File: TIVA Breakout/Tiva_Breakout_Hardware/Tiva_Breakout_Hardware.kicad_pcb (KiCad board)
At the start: 2 copper layers, 141.4 x 70.3 mm, 67 parts, among them U1 TM4C129E_Launchpad

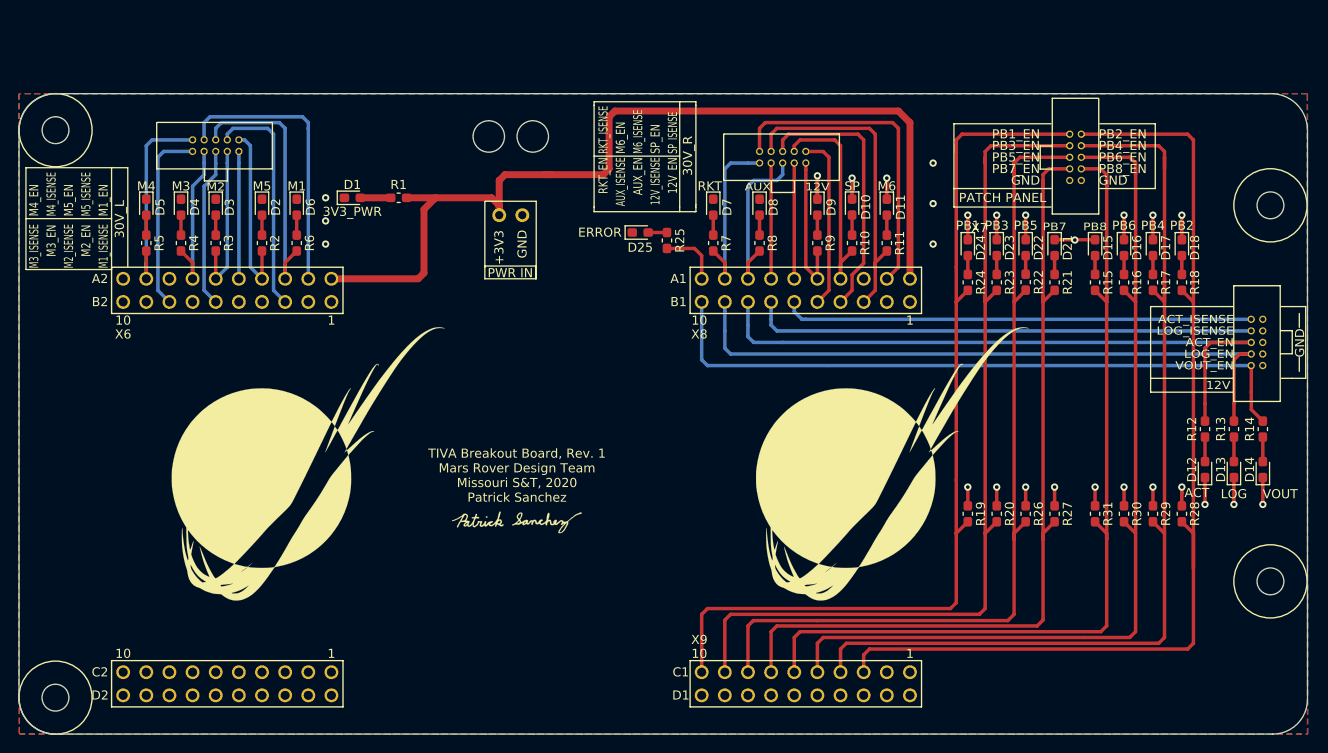
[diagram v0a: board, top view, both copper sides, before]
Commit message: Ready for Board Review, questions about PB#
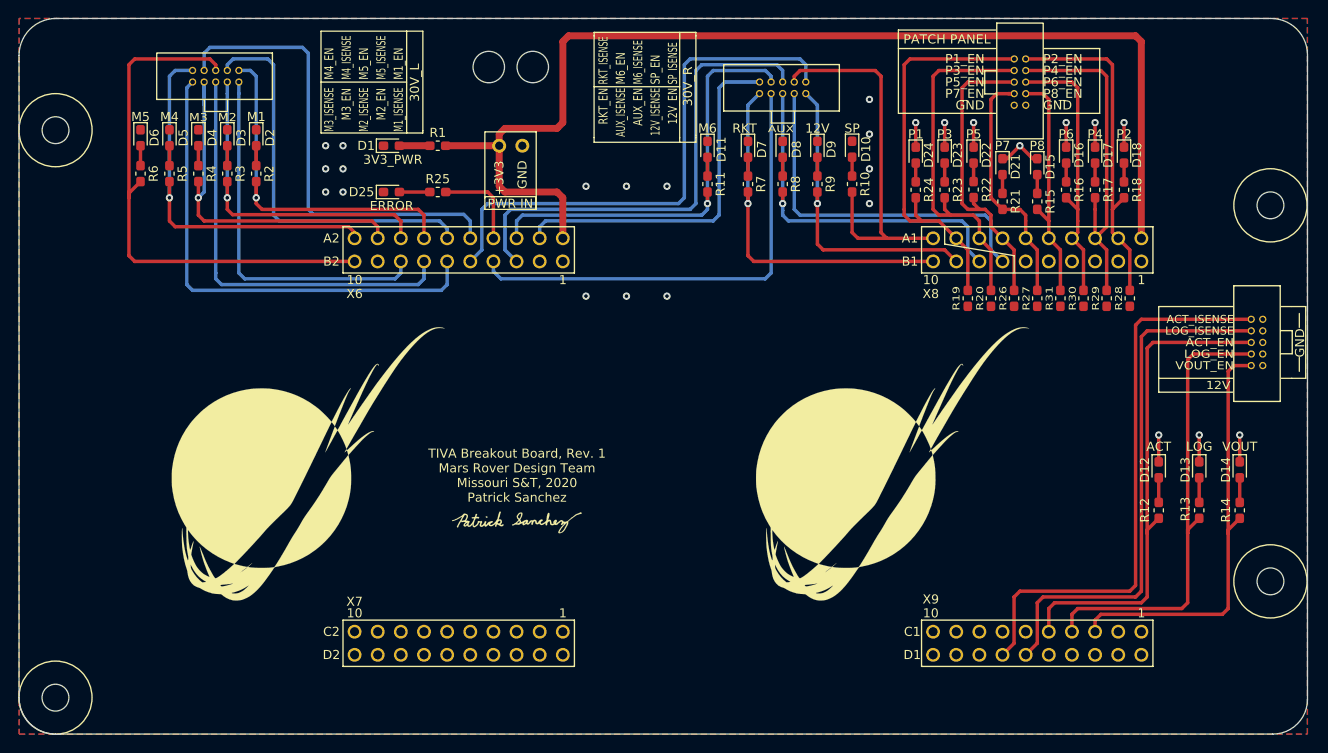
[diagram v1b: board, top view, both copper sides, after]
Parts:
- moved D25 27.7 mm to (125.4, 86.1)
- moved U1 25.8 mm to (209.0, 89.9)
- moved R25 25.7 mm to (130.5, 86.1), turned to 0 degrees
- moved R28 24.3 mm to (206.5, 97.8), turned to 90 degrees
- moved R29 24.2 mm to (203.9, 97.8), turned to 90 degrees
- moved R30 24.1 mm to (201.4, 97.8), turned to 90 degrees
- moved R31 24.0 mm to (198.8, 97.8), turned to 90 degrees
- moved R27 23.7 mm to (196.3, 97.8), turned to 90 degrees
- moved R26 23.7 mm to (193.8, 97.8), turned to 90 degrees
- moved R20 23.7 mm to (191.2, 97.8), turned to 90 degrees
- moved R19 23.7 mm to (188.7, 97.8), turned to 90 degrees
- moved R11 20.7 mm to (160.1, 85.2)
- moved D11 20.7 mm to (160.1, 81.4)
- moved D6 18.8 mm to (97.9, 80.2)
- moved R6 18.8 mm to (97.9, 84.1)
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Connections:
- U1 pad PA5: Net-(U1-PadPA5) -> M5_EN
- U1 pad PA6: ACT_EN -> AUX_EN
- U1 pad PB2: RKT_EN -> PB1_EN
- U1 pad PB3: ERROR -> SP_EN
- U1 pad PB4: M5_ISENSE -> M6_ISENSE
- U1 pad PB5: Net-(U1-PadPB5) -> AUX_ISENSE
- U1 pad PC4: Net-(U1-PadPC4) -> PB4_EN
- U1 pad PC5: SP_EN -> PB6_EN
- U1 pad PC6: 12V_EN -> PB8_EN
- U1 pad PC7: AUX_EN -> PB3_EN
- U1 pad PD0: Net-(U1-PadPD0) -> ACT_ISENSE
- U1 pad PD1: Net-(U1-PadPD1) -> LOG_ISENSE
- U1 pad PD2: M4_ISENSE -> RKT_ISENSE
- U1 pad PD3: AUX_ISENSE -> PB5_EN
- U1 pad PD4: M1_ISENSE -> M4_ISENSE
- U1 pad PD5: M2_EN -> M5_ISENSE
- U1 pad PD7: LOG_ISENSE -> 12V_ISENSE
- U1 pad PE0: M6_EN -> Net-(U1-PadPE0)
- U1 pad PE1: M6_ISENSE -> Net-(U1-PadPE1)
- U1 pad PE2: SP_ISENSE -> Net-(U1-PadPE2)
- U1 pad PE3: ACT_ISENSE -> Net-(U1-PadPE3)
- U1 pad PE4: RKT_ISENSE -> PB2_EN
- U1 pad PE5: 12V_ISENSE -> PB7_EN
- U1 pad PF3: PB2_EN -> VOUT_EN
- U1 pad PG0: PB4_EN -> LOG_EN
- U1 pad PK0: Net-(U1-PadPK0) -> SP_ISENSE
- U1 pad PK1: M2_ISENSE -> M3_ISENSE
- U1 pad PK2: Net-(U1-PadPK2) -> M2_ISENSE
- U1 pad PK3: M3_ISENSE -> M1_ISENSE
- U1 pad PL0: PB7_EN -> Net-(U1-PadPL0)
- U1 pad PL1: PB5_EN -> Net-(U1-PadPL1)
- U1 pad PL2: PB3_EN -> Net-(U1-PadPL2)
- U1 pad PL3: PB1_EN -> Net-(U1-PadPL3)
- U1 pad PL4: PB6_EN -> ACT_EN
- U1 pad PL5: PB8_EN -> Net-(U1-PadPL5)
- U1 pad PM4: LOG_EN -> 12V_EN
- U1 pad PM5: VOUT_EN -> RKT_EN
- U1 pad PN4: Net-(U1-PadPN4) -> M4_EN
- U1 pad PN5: M4_EN -> M3_EN
- U1 pad PP0: M5_EN -> M6_EN
- U1 pad PP1: M1_EN -> ERROR
- U1 pad PP4: Net-(U1-PadPP4) -> M2_EN
- U1 pad PQ0: M3_EN -> M1_EN
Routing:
- net PB2_EN: track 113.8 -> 37.1 mm
- net PB8_EN: track 96.7 -> 26.1 mm
- net PB4_EN: track 108.8 -> 38.1 mm
- net PB6_EN: track 100.5 -> 30.8 mm
- net PB7_EN: track 92.4 -> 27.6 mm
- net PB5_EN: track 95.6 -> 33.3 mm
- net PB3_EN: track 99.4 -> 39.7 mm
- net PB1_EN: track 102.6 -> 44.7 mm
- net SP_ISENSE: track 19.2 -> 59.4 mm
- net AUX_ISENSE: track 12.7 -> 51.9 mm
- net M3_ISENSE: track 20.5 -> 54.1 mm
- net M5_EN: track 29.5 -> 59.0 mm
- net M2_ISENSE: track 17.6 -> 46.9 mm
- net 12V_ISENSE: track 12.7 -> 39.8 mm
- net M1_ISENSE: track 14.0 -> 40.5 mm
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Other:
- board size 141.4 x 70.3 mm -> 141.4 x 78.6 mm
- board text added: "P1"
- board text added: "P1_EN"
- board text added: "P2"
- board text added: "P2_EN"
- board text added: "P3"
- board text added: "P3_EN"
- board text added: "P4"
- board text added: "P4_EN"
- board text added: "P5"
- board text added: "P5_EN"
- board text added: "P6"
- board text added: "P6_EN"
- board text added: "P7"
- board text added: "P7_EN"
- board text added: "P8"
- board text added: "P8_EN"
- board text removed: "PB1"
- board text removed: "PB1_EN"
- board text removed: "PB2"
- board text removed: "PB2_EN"
- board text removed: "PB3"
- board text removed: "PB3_EN"
- board text removed: "PB4"
- board text removed: "PB4_EN"
- board text removed: "PB5"
- board text removed: "PB5_EN"
- board text removed: "PB6"
- board text removed: "PB6_EN"
- board text removed: "PB7"
- board text removed: "PB7_EN"
- board text removed: "PB8"
- board text removed: "PB8_EN"
